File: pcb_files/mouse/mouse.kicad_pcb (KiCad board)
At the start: 2 copper layers, 23 parts, among them Q0 Q_Photo_NPN, Q1 Q_Photo_NPN, Q2 Q_Photo_NPN, Q3 Q_Photo_NPN, U1 Teensy3.2, U2 SN754410NE, U3 LM1084-5.0, U4 Encoder_3081, U5 Encoder_3081, U6 NRF24L01_Breakout

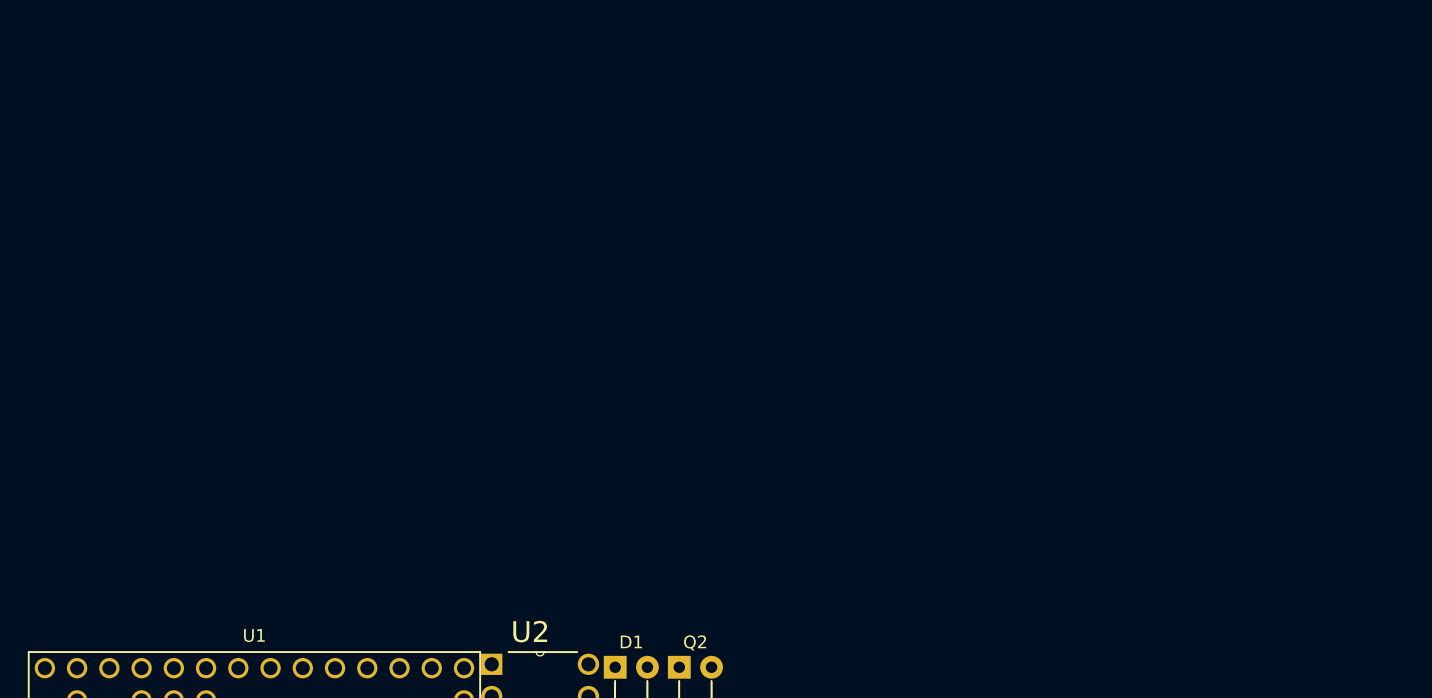
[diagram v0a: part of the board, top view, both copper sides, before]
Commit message: caster ball footprint
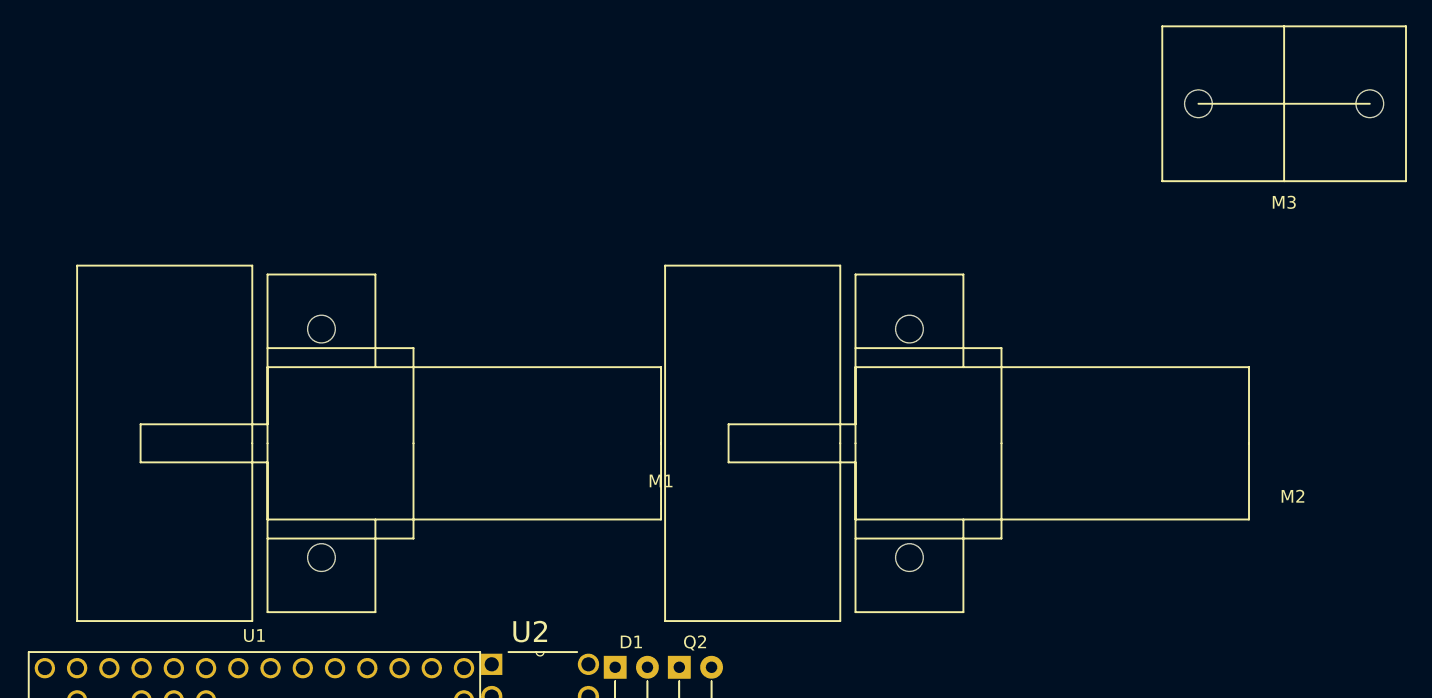
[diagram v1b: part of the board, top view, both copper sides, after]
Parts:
- added M1: Motor_DC, misc:Motor_mouse, F.Cu at (172.7, 77.4)
- added M2: Motor_DC, misc:Motor_mouse, F.Cu at (219.1, 77.4)
- added M3: Motor_DC, misc:Mouse_caster, F.Cu at (221.8, 50.7)
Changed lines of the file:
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@@
     (tracks 0)
     (zones 0)
-    (modules 23)
+    (modules 26)
     (nets 74)
   )
@@
     )
   )
+  (module misc:Motor_mouse (layer F.Cu)
+    (at 172.744801 77.435301)
+    (fp_text reference M1 (at 0 3) (layer F.SilkS)
+      (effects (font (size 1 1) (thickness 0.15)))
+    )
+    (fp_text value Motor_DC (at 0 1.5) (layer F.Fab)
+      (effects (font (size 1 1) (thickness 0.15)))
+    )
+    (fp_line (start 0 0) (end 0 6) (layer F.SilkS) (width 0.15))
+    (fp_line (start 0 0) (end 0 -6) (layer F.SilkS) (width 0.15))
+    (fp_line (start 0 -6) (end -31 -6) (layer F.SilkS) (width 0.15))
+    (fp_line (start 0 6) (end -31 6) (layer F.SilkS) (width 0.15))
+    (fp_line (start -31 -6) (end -31 -1.5) (layer F.SilkS) (width 0.15))
+    (fp_line (start -31 6) (end -31 1.5) (layer F.SilkS) (width 0.15))
+    (fp_line (start -31 -1.5) (end -41 -1.5) (layer F.SilkS) (width 0.15))
+    (fp_line (start -31 1.5) (end -41 1.5) (layer F.SilkS) (width 0.15))
+    (fp_line (start -41 -1.5) (end -41 1.5) (layer F.SilkS) (width 0.15))
+    (fp_line (start -32.2 0) (end -32.2 -14) (layer F.SilkS) (width 0.15))
+    (fp_line (start -32.2 0) (end -32.2 14) (layer F.SilkS) (width 0.15))
+    (fp_line (start -32.2 -14) (end -46 -14) (layer F.SilkS) (width 0.15))
+    (fp_line (start -32.2 14) (end -46 14) (layer F.SilkS) (width 0.15))
+    (fp_line (start -46 -14) (end -46 14) (layer F.SilkS) (width 0.15))
+    (fp_line (start -22.5 6) (end -22.5 13.3) (layer F.SilkS) (width 0.15))
+    (fp_line (start -22.5 -6) (end -22.5 -13.3) (layer F.SilkS) (width 0.15))
+    (fp_line (start -31 0) (end -31 13.3) (layer F.SilkS) (width 0.15))
+    (fp_line (start -31 0) (end -31 -13.3) (layer F.SilkS) (width 0.15))
+    (fp_line (start -31 -13.3) (end -22.5 -13.3) (layer F.SilkS) (width 0.15))
+    (fp_line (start -31 13.3) (end -22.5 13.3) (layer F.SilkS) (width 0.15))
+    (fp_line (start -19.5 0) (end -19.5 7.5) (layer F.SilkS) (width 0.15))
+    (fp_line (start -19.5 0) (end -19.5 -7.5) (layer F.SilkS) (width 0.15))
+    (fp_line (start -31 -7.5) (end -19.5 -7.5) (layer F.SilkS) (width 0.15))
+    (fp_line (start -31 7.5) (end -19.5 7.5) (layer F.SilkS) (width 0.15))
+    (pad "" np_thru_hole circle (at -26.75 -9) (size 2.1844 2.1844) (drill 2.1844) (layers *.Cu *.Mask))
+    (pad "" np_thru_hole circle (at -26.75 9) (size 2.1844 2.1844) (drill 2.1844) (layers *.Cu *.Mask))
+  )
+  (module misc:Motor_mouse (layer F.Cu)
+    (at 219.064801 77.435301)
+    (fp_text reference M2 (at 3.464599 4.212999) (layer F.SilkS)
+      (effects (font (size 1 1) (thickness 0.15)))
+    )
+    (fp_text value Motor_DC (at 0 1.5) (layer F.Fab)
+      (effects (font (size 1 1) (thickness 0.15)))
+    )
+    (fp_line (start -31 7.5) (end -19.5 7.5) (layer F.SilkS) (width 0.15))
+    (fp_line (start -31 -7.5) (end -19.5 -7.5) (layer F.SilkS) (width 0.15))
+    (fp_line (start -19.5 0) (end -19.5 -7.5) (layer F.SilkS) (width 0.15))
+    (fp_line (start -19.5 0) (end -19.5 7.5) (layer F.SilkS) (width 0.15))
+    (fp_line (start -31 13.3) (end -22.5 13.3) (layer F.SilkS) (width 0.15))
+    (fp_line (start -31 -13.3) (end -22.5 -13.3) (layer F.SilkS) (width 0.15))
+    (fp_line (start -31 0) (end -31 -13.3) (layer F.SilkS) (width 0.15))
+    (fp_line (start -31 0) (end -31 13.3) (layer F.SilkS) (width 0.15))
+    (fp_line (start -22.5 -6) (end -22.5 -13.3) (layer F.SilkS) (width 0.15))
+    (fp_line (start -22.5 6) (end -22.5 13.3) (layer F.SilkS) (width 0.15))
+    (fp_line (start -46 -14) (end -46 14) (layer F.SilkS) (width 0.15))
+    (fp_line (start -32.2 14) (end -46 14) (layer F.SilkS) (width 0.15))
+    (fp_line (start -32.2 -14) (end -46 -14) (layer F.SilkS) (width 0.15))
+    (fp_line (start -32.2 0) (end -32.2 14) (layer F.SilkS) (width 0.15))
+    (fp_line (start -32.2 0) (end -32.2 -14) (layer F.SilkS) (width 0.15))
+    (fp_line (start -41 -1.5) (end -41 1.5) (layer F.SilkS) (width 0.15))
+    (fp_line (start -31 1.5) (end -41 1.5) (layer F.SilkS) (width 0.15))
+    (fp_line (start -31 -1.5) (end -41 -1.5) (layer F.SilkS) (width 0.15))
+    (fp_line (start -31 6) (end -31 1.5) (layer F.SilkS) (width 0.15))
+    (fp_line (start -31 -6) (end -31 -1.5) (layer F.SilkS) (width 0.15))
+    (fp_line (start 0 6) (end -31 6) (layer F.SilkS) (width 0.15))
+    (fp_line (start 0 -6) (end -31 -6) (layer F.SilkS) (width 0.15))
+    (fp_line (start 0 0) (end 0 -6) (layer F.SilkS) (width 0.15))
+    (fp_line (start 0 0) (end 0 6) (layer F.SilkS) (width 0.15))
+    (pad "" np_thru_hole circle (at -26.75 9) (size 2.1844 2.1844) (drill 2.1844) (layers *.Cu *.Mask))
+    (pad "" np_thru_hole circle (at -26.75 -9) (size 2.1844 2.1844) (drill 2.1844) (layers *.Cu *.Mask))
+  )
+  (module misc:Mouse_caster (layer F.Cu)
+    (at 221.8309 50.6857)
+    (fp_text reference M3 (at 0 7.8) (layer F.SilkS)
+      (effects (font (size 1 1) (thickness 0.15)))
+    )
+    (fp_text value Motor_DC (at 0.1 9.5) (layer F.Fab)
+      (effects (font (size 1 1) (thickness 0.15)))
+    )
+    (fp_line (start 0 0) (end 6.75 0) (layer F.SilkS) (width 0.15))
+    (fp_line (start 0 0) (end -6.75 0) (layer F.SilkS) (width 0.15))
+    (fp_line (start 0 0) (end 0 -6.1) (layer F.SilkS) (width 0.15))
+    (fp_line (start 0 0) (end 0 6.1) (layer F.SilkS) (width 0.15))
+    (fp_line (start 0 -6.1) (end -9.6 -6.1) (layer F.SilkS) (width 0.15))
+    (fp_line (start 0 -6.1) (end 9.6 -6.1) (layer F.SilkS) (width 0.15))
+    (fp_line (start 0 6.1) (end 9.6 6.1) (layer F.SilkS) (width 0.15))
+    (fp_line (start 0 6.1) (end -9.6 6.1) (layer F.SilkS) (width 0.15))
+    (fp_line (start 9.6 6.1) (end 9.6 -6.1) (layer F.SilkS) (width 0.15))
+    (fp_line (start -9.6 6.1) (end -9.6 -6.1) (layer F.SilkS) (width 0.15))
+    (pad "" np_thru_hole circle (at 6.75 0) (size 2.1844 2.1844) (drill 2.1844) (layers *.Cu *.Mask))
+    (pad "" np_thru_hole circle (at -6.75 0) (size 2.1844 2.1844) (drill 2.1844) (layers *.Cu *.Mask))
+  )
 )

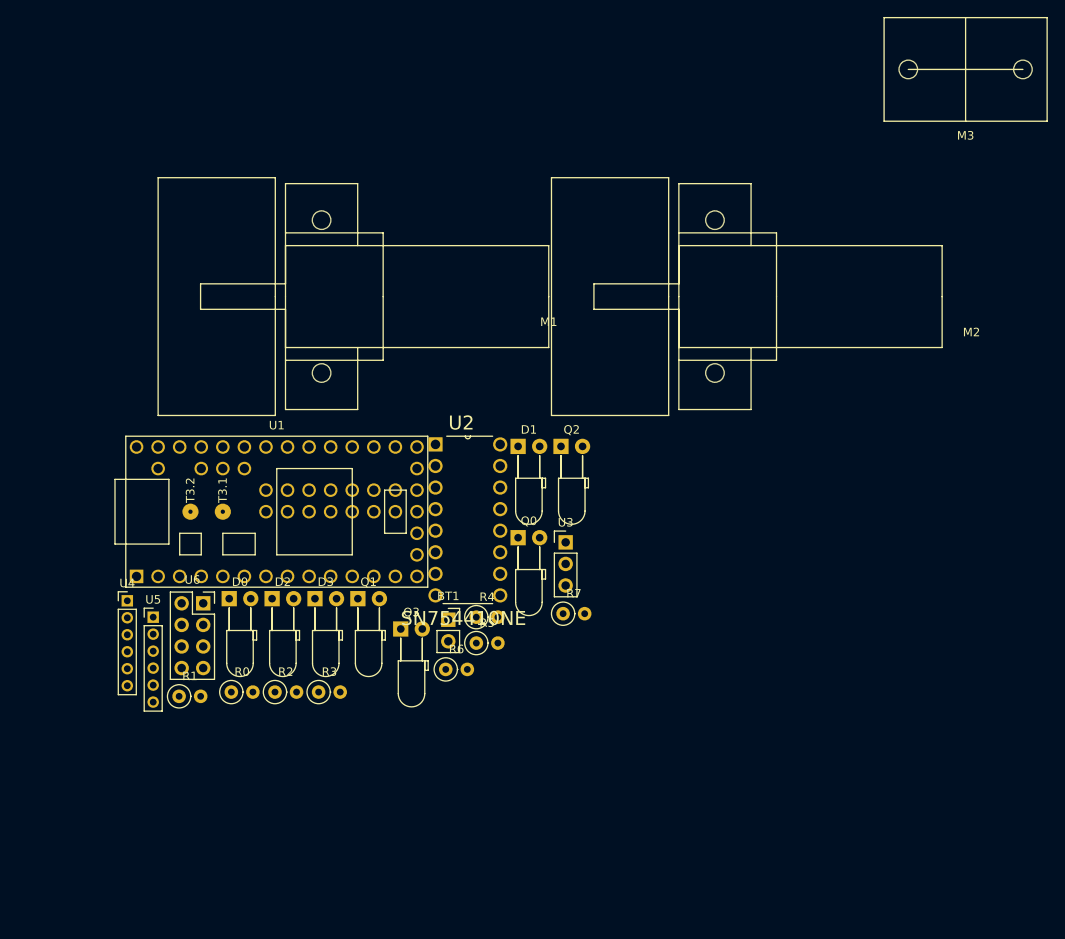
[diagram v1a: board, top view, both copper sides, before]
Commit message: started basic layout
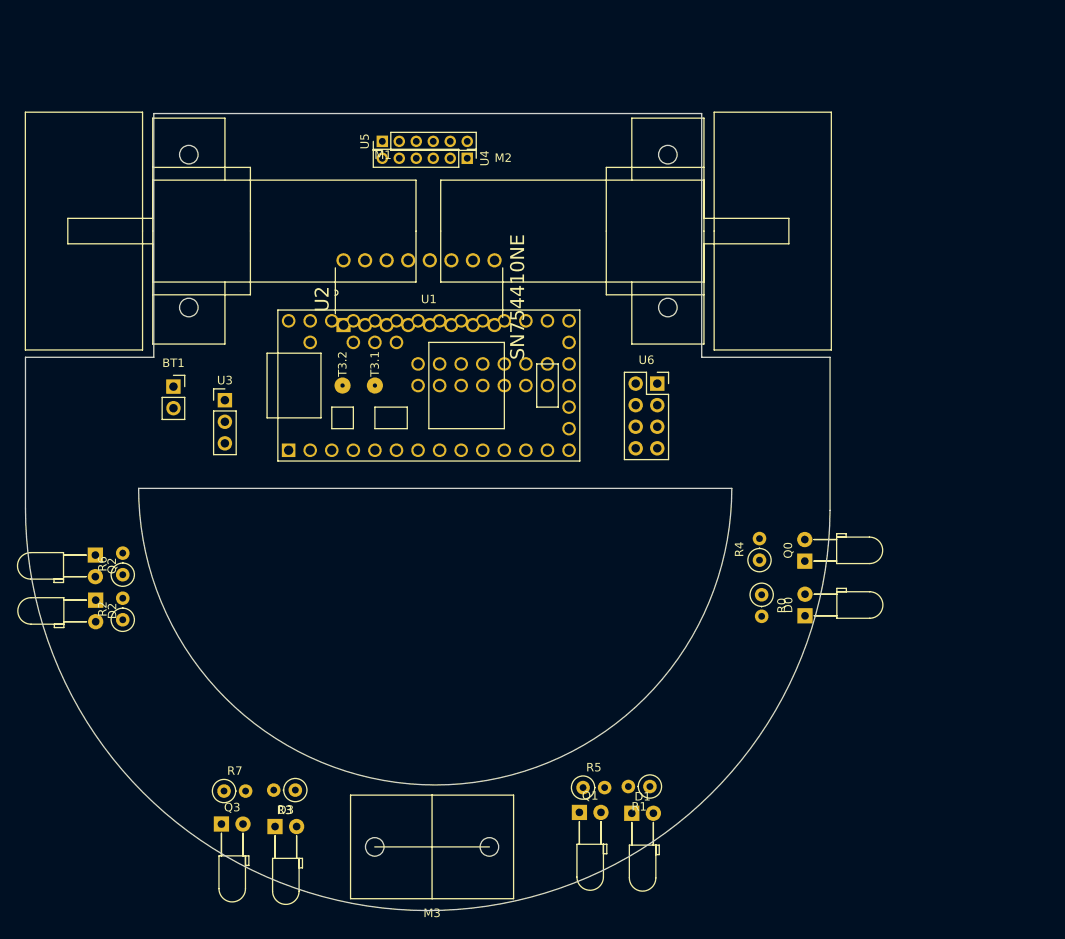
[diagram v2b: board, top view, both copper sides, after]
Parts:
- moved M3 111.0 mm to (159.0, 142.2)
- moved D0 67.8 mm to (202.9, 115.0), turned to 90 degrees
- moved U4 65.7 mm to (163.1, 61.2), turned to 270 degrees
- moved R0 63.5 mm to (197.8, 112.5), turned to 270 degrees
- moved U5 62.2 mm to (153.1, 59.2), turned to 90 degrees
- moved M2 59.5 mm to (160.0, 69.7), turned to 180 degrees
- moved U6 59.4 mm to (185.5, 87.7)
- moved R1 56.5 mm to (184.7, 135.1), turned to 180 degrees
- moved Q2 56.3 mm to (119.4, 107.9), turned to 270 degrees
- moved D1 45.2 mm to (182.5, 138.3)
- moved R7 45.1 mm to (134.5, 135.7)
- moved U3 43.5 mm to (134.6, 89.6)
- moved BT1 42.4 mm to (128.5, 88.0)
- moved R6 39.6 mm to (122.6, 110.2), turned to 90 degrees
- moved U2 39.5 mm to (166.4, 73.2), turned to 90 degrees
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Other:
- board outline added: 94.7 x 93.9 mm
